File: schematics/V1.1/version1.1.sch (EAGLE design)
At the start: 101 parts, among them IC1 ADG1604S, IC2 LM317MBSTT3, IC3 AD8610R, IC4 AD8610R, IC5 337IMP, IC6 AD8620R, Q1 16MHz, T1 BC847, T2 BC847, T3 BC847, T4 BC847, X2 BU-SMA-H

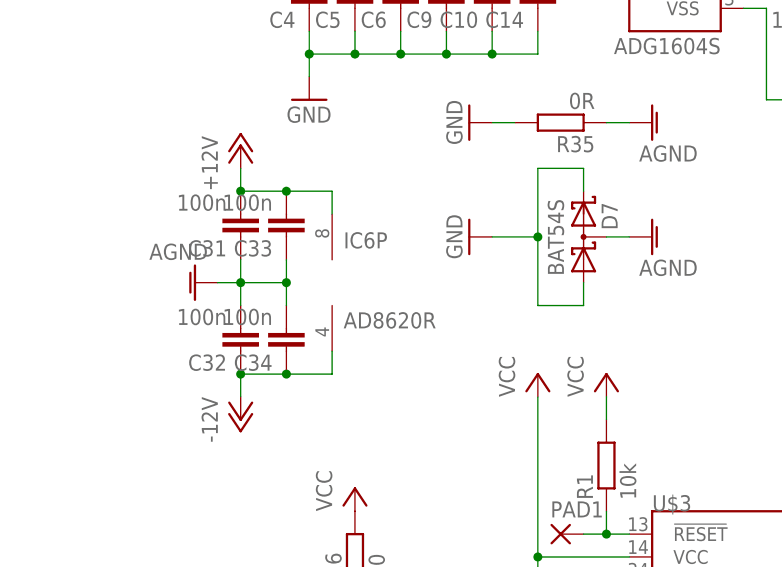
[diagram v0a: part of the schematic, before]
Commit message: finalize the v1.1 layout
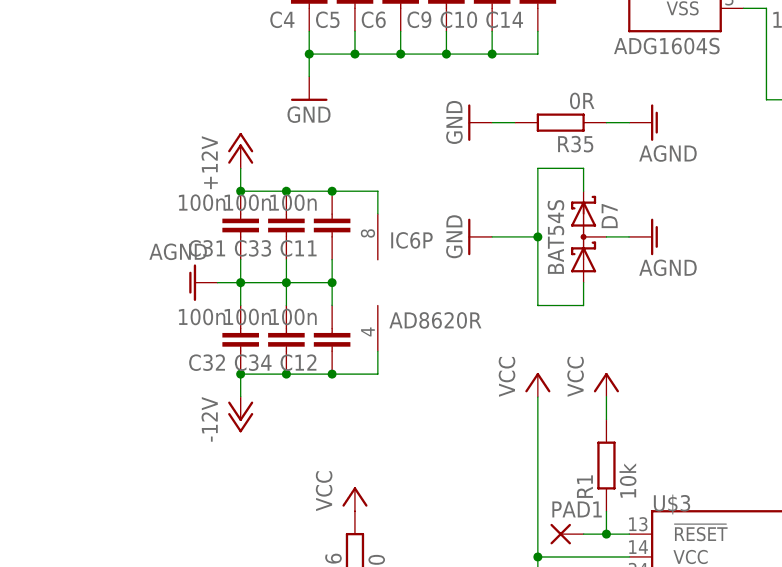
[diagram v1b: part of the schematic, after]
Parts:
- added C11, C12: 100n, rcl:C-EUC0603
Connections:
- net +12V: now also C11.2
- net -12V: now also C12.1
- net AGND: now also C11.1, C12.2
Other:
- moved on the sheet: IC6P
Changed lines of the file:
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@@
 <part name="AGND17" library="supply1" deviceset="AGND" device=""/>
 <part name="GND13" library="supply1" deviceset="GND" device=""/>
+<part name="C11" library="rcl" deviceset="C-EU" device="C0603" value="100n"/>
+<part name="C12" library="rcl" deviceset="C-EU" device="C0603" value="100n"/>
 </parts>
 <sheets>
@@
 <instance part="IC6" gate="A" x="180.34" y="33.02" rot="MR180"/>
 <instance part="IC6" gate="B" x="180.34" y="12.7" rot="MR180"/>
-<instance part="IC6" gate="P" x="5.08" y="132.08"/>
+<instance part="IC6" gate="P" x="10.16" y="132.08"/>
 <instance part="R27" gate="G$1" x="180.34" y="43.18" rot="R180"/>
 <instance part="R28" gate="G$1" x="165.1" y="35.56" rot="R180"/>
@@
 <instance part="AGND17" gate="VR1" x="40.64" y="149.86" rot="R90"/>
 <instance part="GND13" gate="1" x="20.32" y="149.86" rot="R270"/>
+<instance part="C11" gate="G$1" x="5.08" y="137.16" smashed="yes" rot="R180">
+<attribute name="NAME" x="3.556" y="136.779" size="1.778" layer="95" rot="R180"/>
+<attribute name="VALUE" x="3.556" y="141.859" size="1.778" layer="96" rot="R180"/>
+</instance>
+<instance part="C12" gate="G$1" x="5.08" y="124.46" smashed="yes" rot="R180">
+<attribute name="NAME" x="3.556" y="124.079" size="1.778" layer="95" rot="R180"/>
+<attribute name="VALUE" x="3.556" y="129.159" size="1.778" layer="96" rot="R180"/>
+</instance>
 </instances>
 <busses>
@@
 <wire x1="0" y1="129.54" x2="0" y2="132.08" width="0.1524" layer="91"/>
 <junction x="0" y="132.08"/>
+<pinref part="C12" gate="G$1" pin="2"/>
+<pinref part="C11" gate="G$1" pin="1"/>
+<wire x1="5.08" y1="129.54" x2="5.08" y2="132.08" width="0.1524" layer="91"/>
+<wire x1="5.08" y1="132.08" x2="5.08" y2="134.62" width="0.1524" layer="91"/>
+<wire x1="0" y1="132.08" x2="5.08" y2="132.08" width="0.1524" layer="91"/>
+<junction x="5.08" y="132.08"/>
 </segment>
 <segment>
@@
 <junction x="-5.08" y="142.24"/>
 <pinref part="IC6" gate="P" pin="V+"/>
-<wire x1="5.08" y1="139.7" x2="5.08" y2="142.24" width="0.1524" layer="91"/>
+<wire x1="10.16" y1="139.7" x2="10.16" y2="142.24" width="0.1524" layer="91"/>
+<wire x1="10.16" y1="142.24" x2="5.08" y2="142.24" width="0.1524" layer="91"/>
+<junction x="0" y="142.24"/>
+<pinref part="C11" gate="G$1" pin="2"/>
 <wire x1="5.08" y1="142.24" x2="0" y2="142.24" width="0.1524" layer="91"/>
-<junction x="0" y="142.24"/>
+<junction x="5.08" y="142.24"/>
 </segment>
 </net>
@@
 <junction x="-5.08" y="121.92"/>
 <pinref part="IC6" gate="P" pin="V-"/>
-<wire x1="5.08" y1="124.46" x2="5.08" y2="121.92" width="0.1524" layer="91"/>
+<wire x1="10.16" y1="124.46" x2="10.16" y2="121.92" width="0.1524" layer="91"/>
+<wire x1="10.16" y1="121.92" x2="5.08" y2="121.92" width="0.1524" layer="91"/>
+<junction x="0" y="121.92"/>
+<pinref part="C12" gate="G$1" pin="1"/>
 <wire x1="5.08" y1="121.92" x2="0" y2="121.92" width="0.1524" layer="91"/>
-<junction x="0" y="121.92"/>
-</segment>
-</net>
+<junction x="5.08" y="121.92"/>
+</segment>
+</net>
